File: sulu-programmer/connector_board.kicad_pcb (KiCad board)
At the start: 2 copper layers, 40.9 x 33.6 mm, 17 parts, among them J1 Conn_01x08, J2 Conn_01x08, J3 Conn_02x04_Counter_Clockwise, J4 Conn_01x03, J5 Conn_01x02, J6 Conn_01x08, J7 Conn_01x08

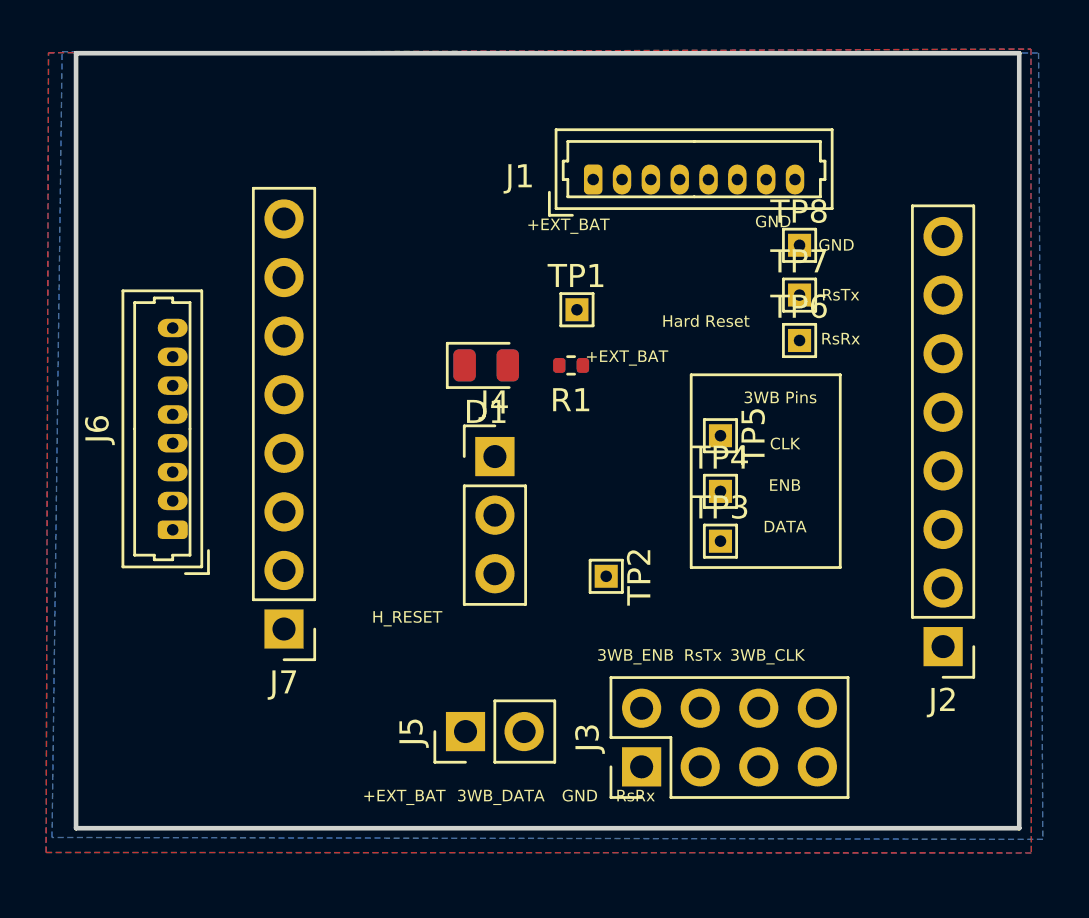
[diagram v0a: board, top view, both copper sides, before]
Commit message: SCuM Programmer Rev. 2, submitted for fab
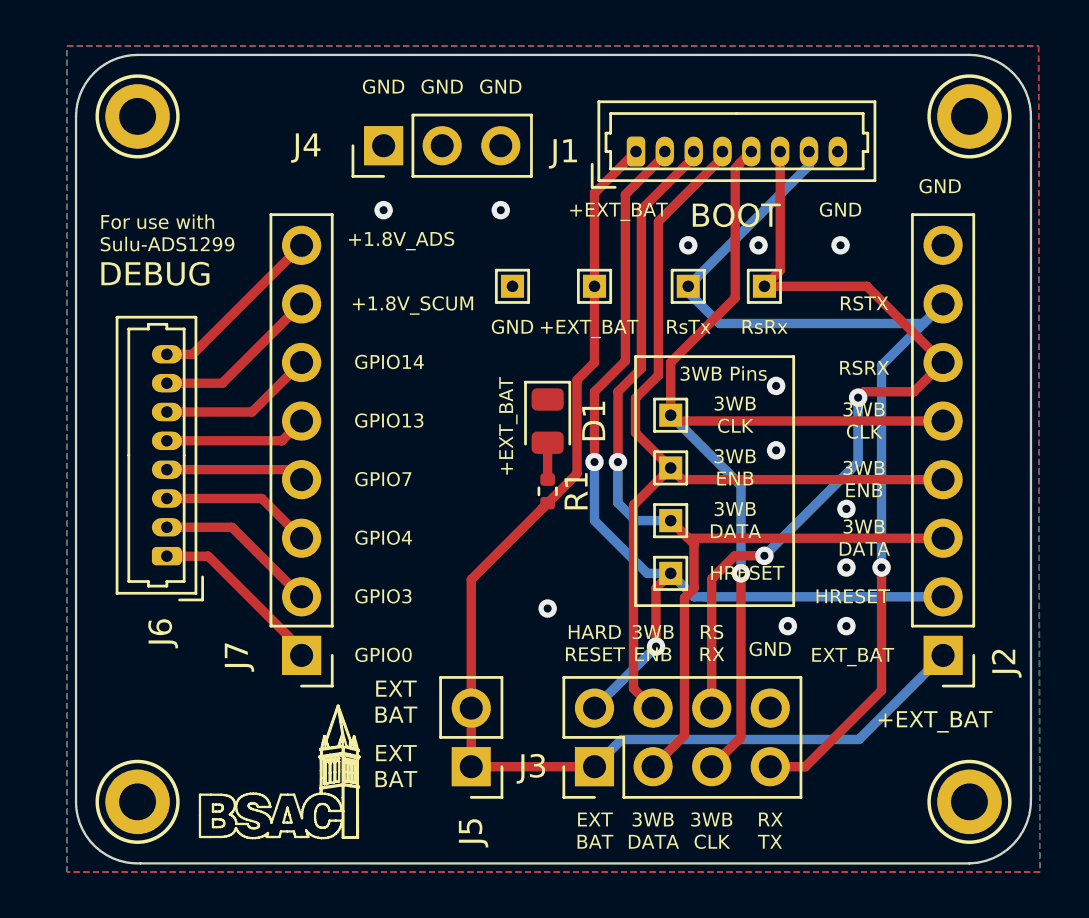
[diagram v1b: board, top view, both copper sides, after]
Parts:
- added TP10: TestPoint, TestPoint:TestPoint_Keystone_5010-5014_Multipurpose, F.Cu at (73.2, 83.1)
- added TP11: TestPoint, TestPoint:TestPoint_Keystone_5010-5014_Multipurpose, F.Cu at (109.2, 53.3)
- added TP12: TestPoint, TestPoint:TestPoint_Keystone_5010-5014_Multipurpose, F.Cu at (109.2, 83.1)
- added TP9: TestPoint, TestPoint:TestPoint_Keystone_5010-5014_Multipurpose, F.Cu at (73.2, 53.3)
- R1: value 100 -> 300
- moved J4 14.3 mm to (83.8, 54.6), turned to 90 degrees
- moved TP8 12.6 mm to (89.4, 60.7)
- moved R1 5.55 mm to (90.9, 69.6), turned to 90 degrees
- moved TP7 4.84 mm to (97.0, 60.7)
- moved D1 3.60 mm to (90.9, 66.5), turned to -90 degrees
- moved TP6 2.80 mm to (100.3, 60.7)
- moved TP2 2.80 mm to (96.3, 73.2), turned to 0 degrees
- moved TP4 2.39 mm to (96.3, 68.6)
- moved TP5 2.33 mm to (96.3, 66.3)
- moved TP3 2.33 mm to (96.3, 70.9)
- moved J1 2.22 mm to (94.8, 54.9)
- moved J3 2.04 mm to (93.0, 81.5)
- moved J5 1.54 mm to (87.6, 81.5), turned to 180 degrees
- moved J7 1.37 mm to (80.3, 76.7)
- moved TP1 1.27 mm to (93.0, 60.7)
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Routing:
- net /+EXT_BAT: track 0.00 -> 52.4 mm
- net /RsTx: track 0.00 -> 44.3 mm, vias 0 -> 1
- net /3WB_DATA: track 0.00 -> 43.2 mm, vias 0 -> 1
- net /3WB_CLK: track 0.00 -> 41.8 mm, vias 0 -> 1
- net /HARD_RESET: track 0.00 -> 41.0 mm, vias 0 -> 2
- net /3WB_ENB: track 0.00 -> 39.4 mm
- net /RsRx: track 0.00 -> 36.4 mm, vias 0 -> 2
- net /+1.8V_ADS: track 0.00 -> 7.80 mm
- net /SCUM_GPIO0: track 0.00 -> 7.77 mm
- net /+1.8V_SCUM: track 0.00 -> 7.27 mm
- net /SCUM_GPIO3: track 0.00 -> 7.09 mm
- net /SCUM_GPIO14: track 0.00 -> 6.73 mm
- net /SCUM_GPIO4: track 0.00 -> 6.56 mm
- net /SCUM_GPIO13: track 0.00 -> 6.20 mm
- net /SCUM_GPIO7: track 0.00 -> 6.02 mm
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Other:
- board size 40.9 x 33.6 mm -> 41.4 x 35.1 mm
- board text added: "+1.8V_ADS"
- board text added: "+1.8V_SCUM"
- board text added: "3WB CLK"
- board text added: "3WB DATA"
- board text added: "3WB ENB"
- board text added: "BOOT"
- board text added: "Berkeley Autonomous Microsystems Lab SCuM Programmer Rev. 2"
- board text added: "DEBUG"
- board text added: "EXT BAT"
- board text added: "EXT_BAT"
- board text added: "For use with Sulu-ADS1299"
- board text added: "GPIO0"
- board text added: "GPIO13"
- board text added: "GPIO14"
- board text added: "GPIO3"
- board text added: "GPIO4"
- board text added: "GPIO7"
- board text added: "HARD RESET"
- board text added: "HRESET"
- board text added: "RS RX"
- board text added: "RSRX"
- board text added: "RSTX"
- board text added: "RX TX"
- board text removed: "3WB_CLK"
- board text removed: "3WB_DATA"
- board text removed: "3WB_ENB"
- board text removed: "CLK"
- board text removed: "DATA"
- board text removed: "ENB"
- board text removed: "H_RESET"
- board text removed: "Hard Reset"
